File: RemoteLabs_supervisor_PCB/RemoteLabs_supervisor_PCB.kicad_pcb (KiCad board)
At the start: 4 copper layers, 182.6 x 99.2 mm, 199 parts, among them J1 Super_Prog_Header, J10 ShiftReg_Header, J11 SPI Student, J12 MCU_Header, J13 USB_B_Mini, J14 ShiftReg_Header, J15 SPI Supervisor, J16 MotorController_PWR_IP, J17 MotorController, J18 DC Motor Output, J19 Stepper Motor Output, J2 WS2821B Header, J20 Servo_A, J21 Servo_B, J22 Thermocouple A, J23 limit_switch_A, J24 limit_switch_B, J25 Optical Encoder, J26 Student_Prog_Header, J27 Analog Buffer, J28 student_PA03, J29 3V3 PWR SRC, J3 XT60_60A_male, J30 12V_DC, J31 5V_DC_RPI, J32 GND_BUS, J33 12V_BUS, J34 5V_P_BUS, J35 5V_D_BUS, J36 3V3_BUS, J4 Strip Lighting, J5 USB_A_Stacked, J6 5V_DC_LED, J7 USB_B_Mini, J8 MCU_Header, J9 Spare Student GPIOs, Q1 IRF5305_PBF, SW1 Stepper_Mode, SW2 Student Reset, SW3 Supervisor Reset, U1 R-78C5.0-1.0, U10 4081, U11 4081, U12 4081, U13 74HC86, U14 74HC86, U15 NCS20074D, U16 NCS20074D, U17 NCS20074D, U18 R-78C5.0-1.0, U19 AD8497, U2 TCYSH14F, U20 74LS07, U21 74LS07, U22 74LS07, U23 TCYSH14F, U3 AMS1117-3.3, U4 ATSAMD21G18A-M, U5 4094, U6 ATSAMD21G18A-M, U7 4094, U8 4069, U9 4081, X1 ASEK-xxxMHz, X2 ASEK-xxxMHz

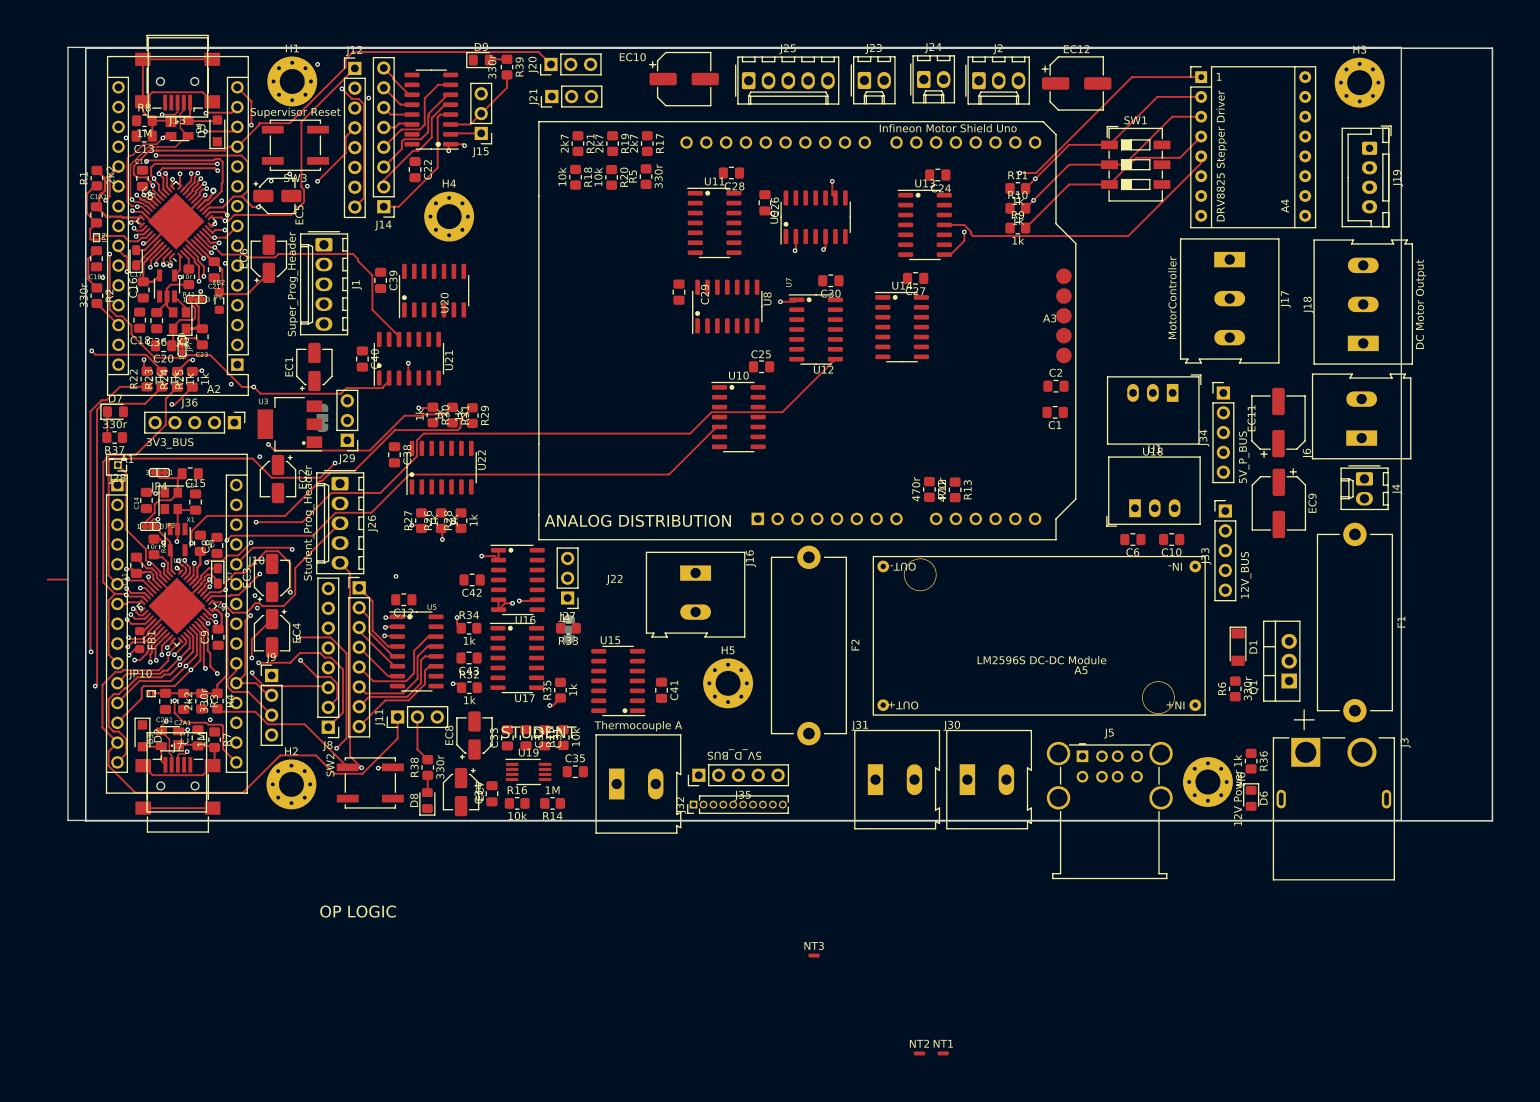
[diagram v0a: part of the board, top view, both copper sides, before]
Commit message: Version 2 PCB Layout
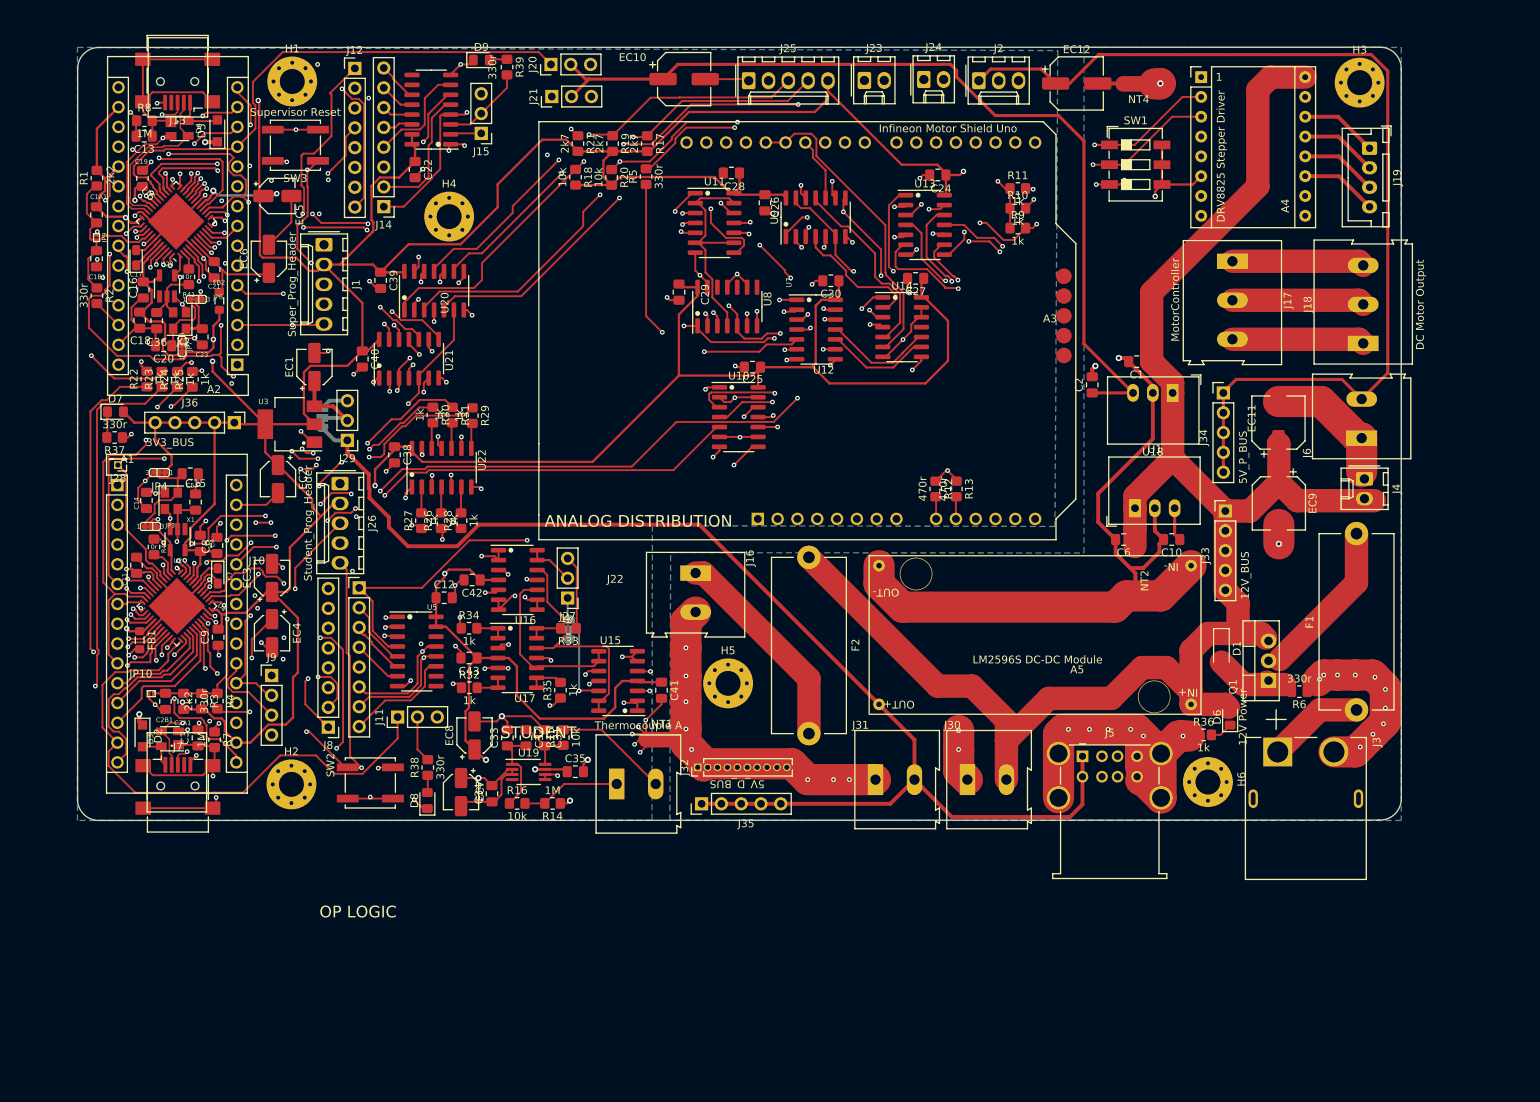
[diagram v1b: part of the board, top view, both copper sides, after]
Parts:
- removed NT3: NetTie, NetTie:NetTie-2_SMD_Pad0.5mm
- added NT4: NetTie_2, NetTie:NetTie-2_SMD_Pad2.0mm, F.Cu at (185.8, 27.4)
- NT1: footprint NetTie:NetTie-2_SMD_Pad0.5mm -> NetTie:NetTie-2_SMD_Pad2.0mm
- moved NT2 66.6 mm to (185.4, 91.1), turned to -90 degrees
- moved NT1 54.1 mm to (124.6, 111.5)
- moved F1 22.5 mm to (213.7, 107.7), turned to 90 degrees
- moved C1 12.3 mm to (185.5, 63.0)
- moved D6 10.8 mm to (197.5, 108.6), turned to 90 degrees
- moved R6 8.22 mm to (206.4, 105.4), turned to 180 degrees
- moved R36 6.96 mm to (194.1, 110.9), turned to 0 degrees
- moved C12 5.18 mm to (96.7, 93.3), turned to 0 degrees
- moved J32 4.80 mm to (129.3, 115.1)
- moved C2 4.65 mm to (179.8, 66.0), turned to 90 degrees
- moved J35 3.67 mm to (129.7, 119.7)
- moved J3 3.59 mm to (207.2, 119.1)
- moved Q1 2.64 mm to (202.4, 103.9)
- moved D1 2.14 mm to (196.4, 99.8)
- moved C6 1.18 mm to (183.9, 85.9)
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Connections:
- A4 pad 9: GNDD -> GNDPWR
- C1 pad 2: GNDD -> GND_PB
- C10 pad 2: GNDD -> GND_PB
- C2 pad 2: GNDD -> GND_PB
- C31 pad 1: GNDA -> GNDD
- C33 pad 2: GNDA -> GNDD
- C34 pad 1: GNDA -> GNDD
- C34 pad 2: GNDA -> GNDD
- C35 pad 2: GNDA -> GNDD
- C6 pad 2: GNDD -> GND_PB
- EC12 pad 2: GNDD -> /Power Input & Distribution/PGND0
- EC7 pad 1: GNDA -> GNDD
- EC7 pad 2: GNDA -> GNDD
- EC8 pad 2: GNDA -> GNDD
- J6 pad 1: GNDD -> GNDPWR
- NT1 pad 1: GND -> GNDD
- NT1 pad 2: GNDD -> GNDPWR
- NT2 pad 1: GND -> GND_PB
- R14 pad 1: GNDA -> GNDD
- U1 pad 2: GNDD -> GND_PB
- U18 pad 2: GNDD -> GND_PB
- U19 pad 2: GNDA -> GNDD
- U19 pad 3: GNDA -> GNDD
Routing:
- net 3V3_DC_MCU: track 33.7 -> 759.7 mm, vias 1 -> 15
- net /Student MCU/DC_MOTOR_DIR1: track 557.3 -> 88.8 mm, vias 2 -> 1
- net 12V_DC_BUS: track 0.00 -> 219.6 mm
- net GNDD: track 60.5 -> 265.7 mm, vias 5 -> 68
- net GNDPWR: track 0.00 -> 180.1 mm, vias 0 -> 28
- net 5V_DC_RPI: track 0.00 -> 162.2 mm
- net 5V_DC_LED: track 0.00 -> 150.0 mm
- net USB_BUS: track 0.00 -> 148.8 mm, vias 0 -> 2
- net STPPR_FAULT: track 0.00 -> 121.7 mm, vias 0 -> 3
- net 5V_DC_SERVO: track 0.00 -> 115.2 mm
- net MODE_2: track 79.2 -> 172.4 mm, vias 3 -> 7
- net /Output Logic/SUPERVISOR_PIXEL_DATA: track 5.17 -> 89.5 mm, vias 1 -> 5
- net /Output Logic/MCU_STEP_SELECT: track 14.3 -> 95.6 mm, vias 0 -> 4
- net /Digital Sensor Buffers/D_IN_B: track 0.00 -> 80.4 mm, vias 0 -> 3
- net /Digital Sensor Buffers/D_IN_A: track 0.00 -> 73.0 mm, vias 0 -> 3
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- added copper zone on B.Cu, net GNDD
- added copper zone on B.Cu, net GNDPWR
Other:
- board size 182.6 x 99.2 mm -> 169.7 x 99.1 mm
